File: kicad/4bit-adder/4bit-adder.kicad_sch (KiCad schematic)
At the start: 69 parts, among them J1 Screw_Terminal_01x02, K1 SR11-5V-200-2C-PH, K10 SR11-5V-200-2C-PH, K11 SR11-5V-200-2C-PH, K12 SR11-5V-200-2C-PH, K13 SR11-5V-200-2C-PH, K14 SR11-5V-200-2C-PH, K15 SR11-5V-200-2C-PH, K16 SR11-5V-200-2C-PH, K17 SR11-5V-200-2C-PH, K18 SR11-5V-200-2C-PH, K19 SR11-5V-200-2C-PH, K2 SR11-5V-200-2C-PH, K20 SR11-5V-200-2C-PH, K21 SR11-5V-200-2C-PH, K22 SR11-5V-200-2C-PH, K23 SR11-5V-200-2C-PH, K24 SR11-5V-200-2C-PH, K3 SR11-5V-200-2C-PH, K4 SR11-5V-200-2C-PH, K5 SR11-5V-200-2C-PH, K6 SR11-5V-200-2C-PH, K7 SR11-5V-200-2C-PH, K8 SR11-5V-200-2C-PH, K9 SR11-5V-200-2C-PH, SW1 SW_Wuerth_450301014042, SW3 A, SW4 B

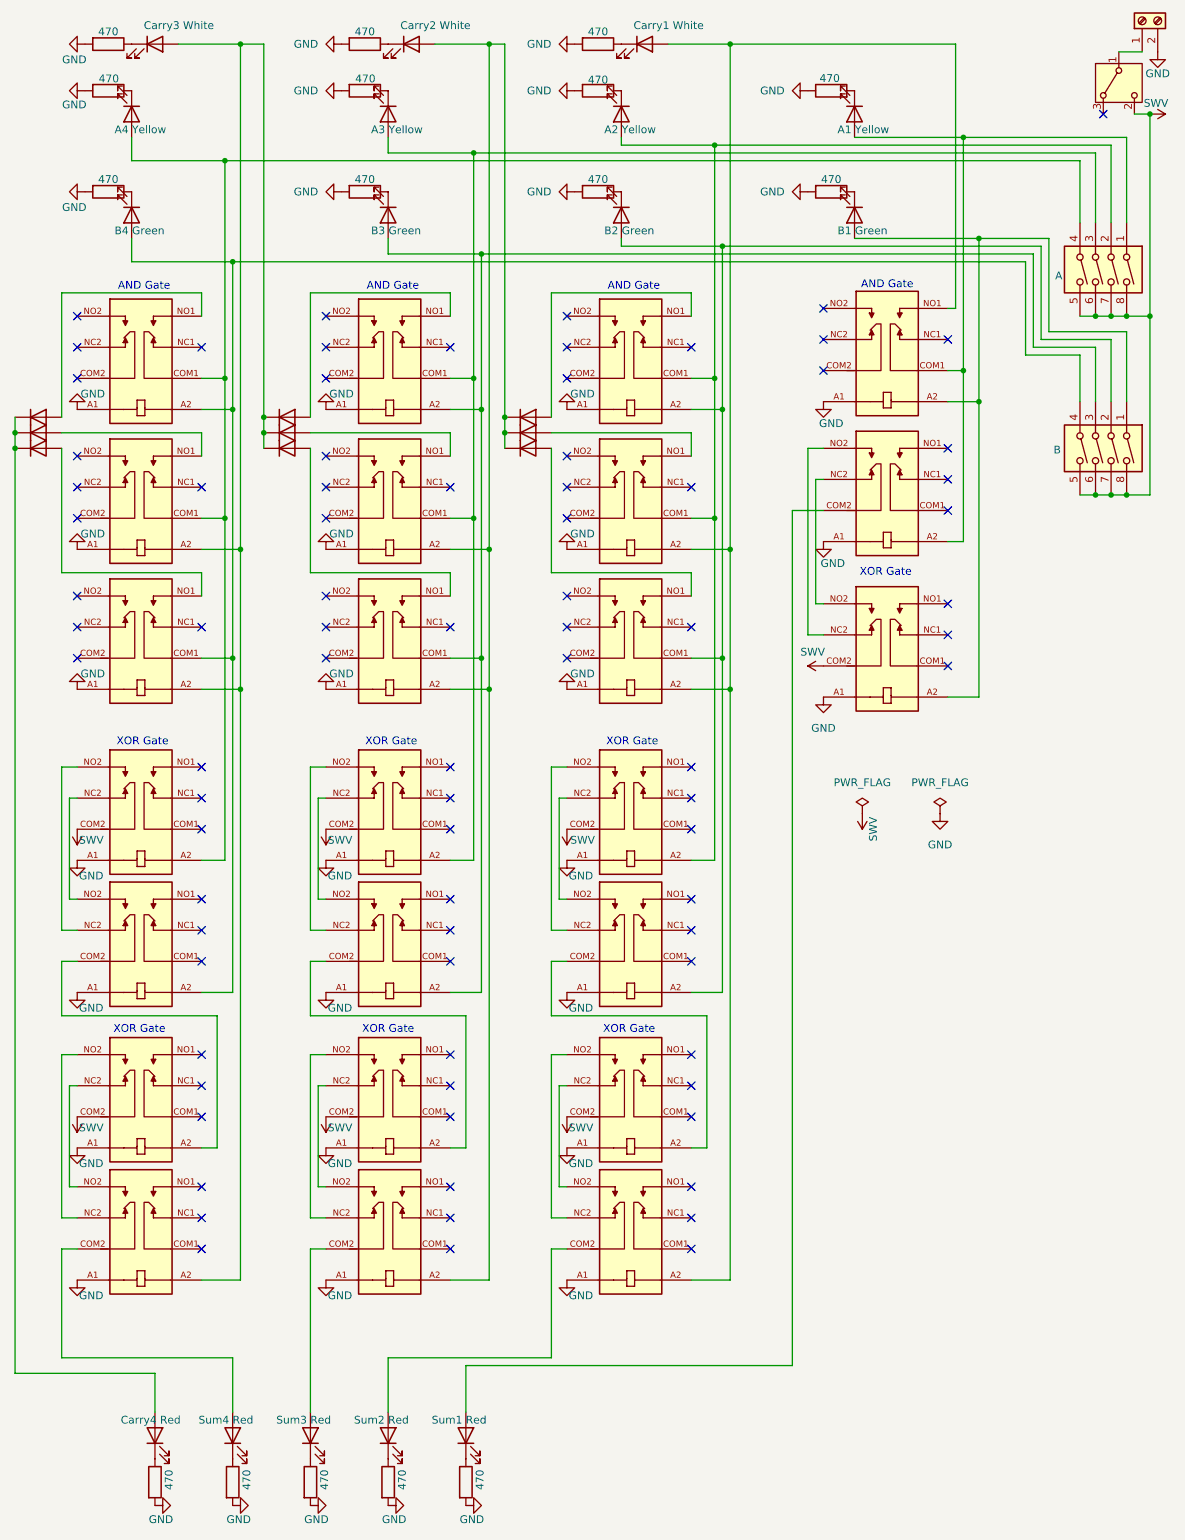
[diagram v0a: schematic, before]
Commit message: footprints initial layout
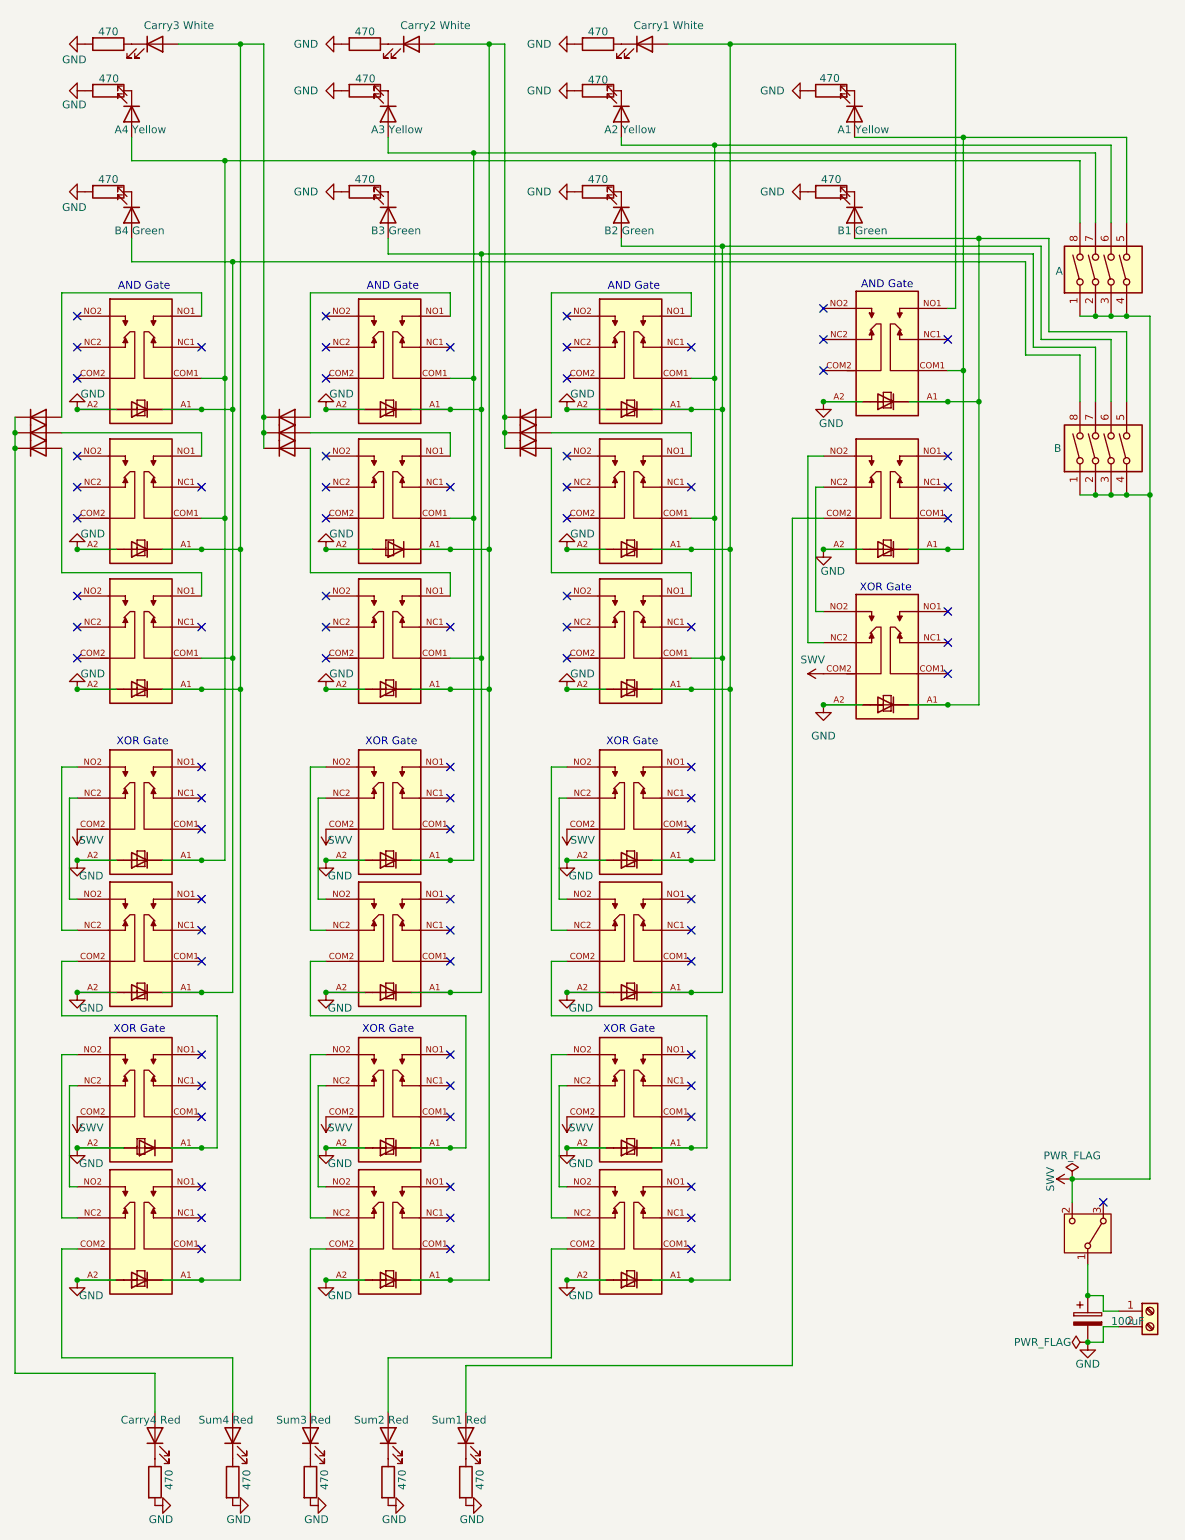
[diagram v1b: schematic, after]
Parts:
- added C1: 100uF, Capacitor_THT:CP_Radial_D10.0mm_P2.50mm, symbol Device:C_Polarized
- added D26, D27, D28, D29, D30, D31, D32, D33, D34, D35, D36, D37, D38, D39, D40, D41, D42, D43, D44, D45, D46, D47, D48, D49: 1N4001, Diode_THT:D_DO-41_SOD81_P10.16mm_Horizontal, symbol Diode:1N4003
- D1, D22, D23, D24, D3, D4, D5, D6, D7: value 1N4007 -> 1N4001
- D10, D11, D12, D13, D14, D15, D16, D17, D18, D19, D2, D20, D21, D25, D8, D9: footprint LED_THT:LED_D5.0mm -> LED_THT:LED_D3.0mm
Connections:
- net GND: now also K1.A2, K10.A2, K11.A2, K12.A2, K13.A2, K14.A2, K15.A2, K16.A2, K17.A2, K18.A2, K19.A2, K2.A2, K20.A2, K21.A2, K22.A2, K23.A2, K24.A2, K3.A2, K4.A2, K5.A2, K6.A2, K7.A2, K8.A2, K9.A2, C1.2, D26.2 (A), D27.2 (A), D28.2 (A), D29.2 (A), D30.2 (A), D31.2 (A), D32.2 (A), D33.2 (A), D34.2 (A), D35.2 (A), D36.2 (A), D37.2 (A), D38.2 (A), D39.2 (A), D40.2 (A), D41.2 (A), D42.2 (A), D43.2 (A), D44.2 (A), D45.2 (A), D46.2 (A), D47.2 (A), D48.2 (A), D49.2 (A); no longer K1.A1, K10.A1, K11.A1, K12.A1, K13.A1, K14.A1, K15.A1, K16.A1, K17.A1, K18.A1, K19.A1, K2.A1, K20.A1, K21.A1, K22.A1, K23.A1, K24.A1, K3.A1, K4.A1, K5.A1, K6.A1, K7.A1, K8.A1, K9.A1
- net SWV: now also SW3.1, SW3.2, SW3.3, SW3.4, SW4.1, SW4.2, SW4.3, SW4.4; no longer SW3.5, SW3.6, SW3.7, SW3.8, SW4.5, SW4.6, SW4.7, SW4.8
- net at D12.2 (A), D5.1 (K), D6.1 (K)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: now also K19.A1, K20.A1, K24.A1, D36.1 (K), D43.1 (K), D46.1 (K); no longer K19.A2, K20.A2, K24.A2
- net at D10.2 (A), K16.COM1, K19.COM1: now also K21.A1, SW3.8, D42.1 (K); no longer K21.A2, SW3.4
- net at D1.1 (K), D11.2 (A), D3.1 (K)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: now also K11.A1, K12.A1, K18.A1, D35.1 (K), D44.1 (K), D45.1 (K); no longer K11.A2, K12.A2, K18.A2
- net at K5.COM2: now also K6.A1, D49.1 (K); no longer K6.A2
- net at K14.COM2: now also K15.A1, D38.1 (K); no longer K15.A2
- net at J1.1 (Pin_1), SW1.1 (B): now also C1.1
- net at D18.2 (A), K1.COM1, K2.COM1: now also K4.A1, SW3.6, D32.1 (K); no longer K4.A2, SW3.2
- net at D16.2 (A), K10.COM1, K11.COM1: now also K13.A1, SW3.7, D41.1 (K); no longer K13.A2, SW3.3
- net at K22.COM2: now also K23.A1, D37.1 (K); no longer K23.A2
- net at D2.2 (A), K7.COM1: now also K8.A1, SW3.5, D27.1 (K); no longer K8.A2, SW3.1
- new net: D15.2 (A), D40.1 (K), D47.1 (K), K16.A1, K20.COM1, K22.A1, SW4.8
- new net: D19.2 (A), D29.1 (K), D33.1 (K), K1.A1, K3.COM1, K5.A1, SW4.6
- new net: D17.2 (A), D39.1 (K), D48.1 (K), K10.A1, K12.COM1, K14.A1, SW4.7
- new net: D30.1 (K), D31.1 (K), D34.1 (K), D9.2 (A), K17.A1, K2.A1, K3.A1, K7.NO1
- new net: D21.2 (A), D26.1 (K), D28.1 (K), K7.A1, K9.A1, SW4.5
